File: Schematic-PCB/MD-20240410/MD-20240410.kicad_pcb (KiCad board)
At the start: 2 copper layers, 100.5 x 56.4 mm, 0 parts

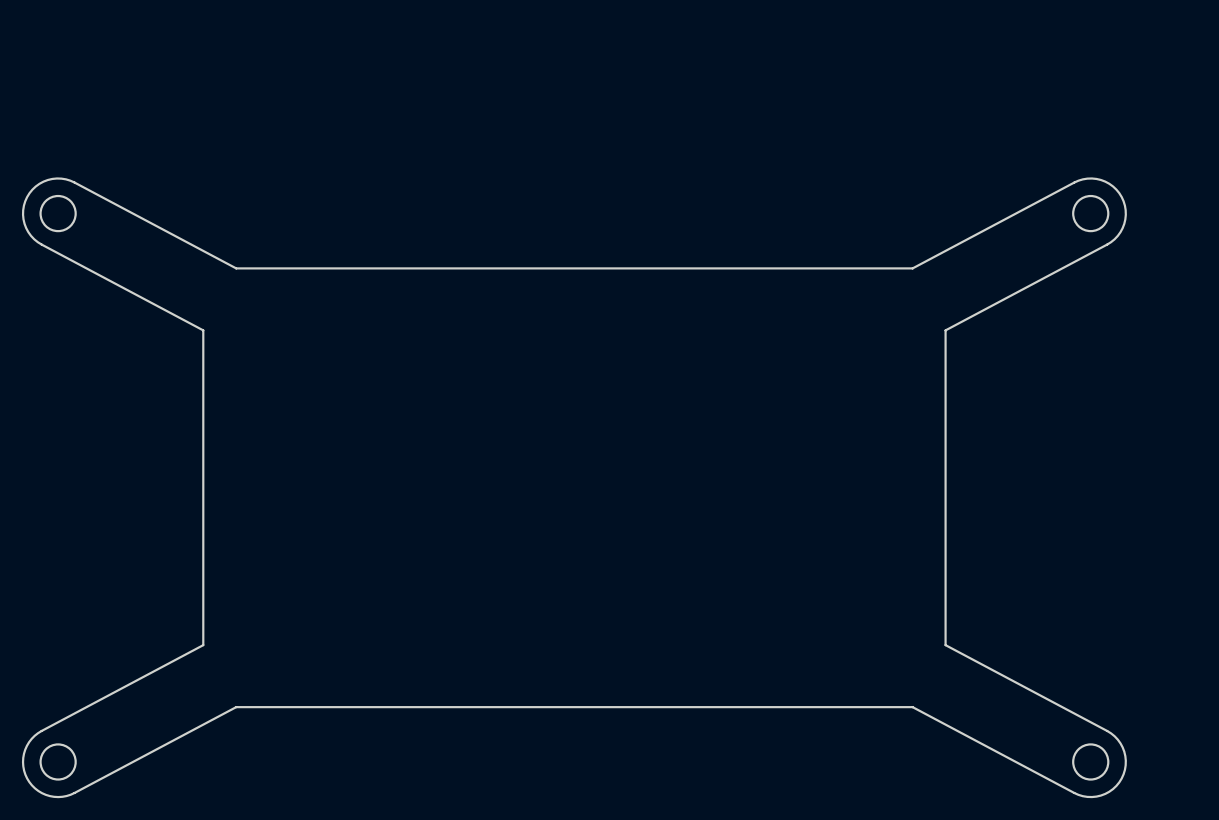
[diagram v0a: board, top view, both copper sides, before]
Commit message: MD基板へ部品を仮で配置
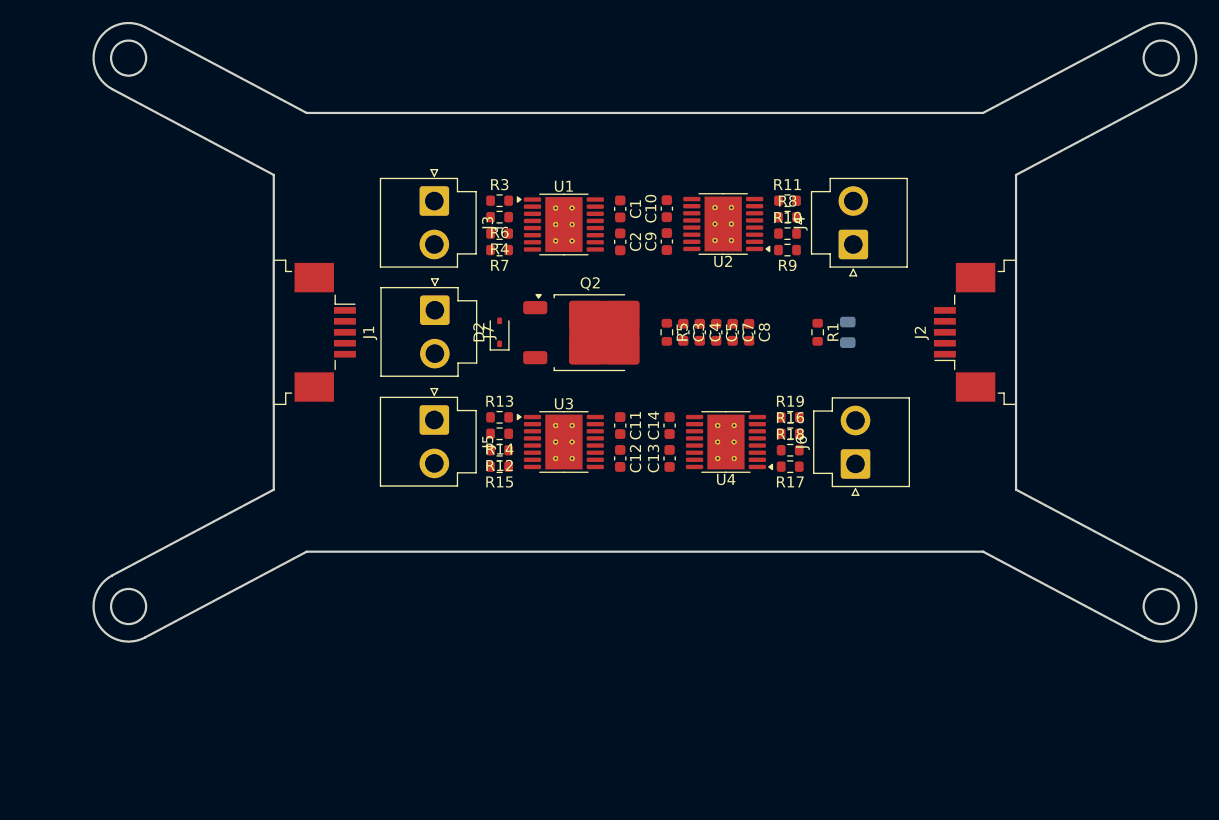
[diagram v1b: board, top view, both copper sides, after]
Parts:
- added C1: 22n, Capacitor_SMD:C_0603_1608Metric, F.Cu at (147.8, 76.2)
- added C10: 220n, Capacitor_SMD:C_0603_1608Metric, F.Cu at (152.0, 76.2)
- added C11: 22n, Capacitor_SMD:C_0603_1608Metric, F.Cu at (147.8, 96.0)
- added C12: 220n, Capacitor_SMD:C_0603_1608Metric, F.Cu at (147.8, 99.0)
- added C13: 22n, Capacitor_SMD:C_0603_1608Metric, F.Cu at (152.2, 99.0)
- added C14: 220n, Capacitor_SMD:C_0603_1608Metric, F.Cu at (152.2, 96.0)
- added C2: 220n, Capacitor_SMD:C_0603_1608Metric, F.Cu at (147.8, 79.2)
- added C3: 4.7u, Capacitor_SMD:C_0603_1608Metric, F.Cu at (153.5, 87.5)
- added C4: 4.7u, Capacitor_SMD:C_0603_1608Metric, F.Cu at (155.0, 87.5)
- added C5: 50u, Capacitor_SMD:C_0603_1608Metric, F.Cu at (156.5, 87.5)
- added C7: 0.1u, Capacitor_SMD:C_0603_1608Metric, F.Cu at (158.0, 87.5)
- added C8: 0.1u, Capacitor_SMD:C_0603_1608Metric, F.Cu at (159.5, 87.5)
- added C9: 22n, Capacitor_SMD:C_0603_1608Metric, F.Cu at (152.0, 79.2)
- added D1: LED, LED_SMD:LED_0805_2012Metric, B.Cu at (168.5, 87.5)
- added D2: 16.2V, Diode_SMD:D_SOD-323, F.Cu at (136.8, 87.5)
- added J1: Conn_01x05_Pin, Connector_FFC-FPC:TE_84953-5_1x05-1MP_P1.0mm_Horizontal, F.Cu at (120.8, 87.5)
- added J2: Conn_01x05_Pin, Connector_FFC-FPC:TE_84953-5_1x05-1MP_P1.0mm_Horizontal, F.Cu at (179.2, 87.5)
- added J3: Conn_01x02_Pin, Connector_JST:JST_VH_B2P-VH_1x02_P3.96mm_Vertical, F.Cu at (130.8, 75.5)
- added J4: Conn_01x02_Pin, Connector_JST:JST_VH_B2P-VH_1x02_P3.96mm_Vertical, F.Cu at (169.0, 79.5)
- added J5: Conn_01x02_Pin, Connector_JST:JST_VH_B2P-VH_1x02_P3.96mm_Vertical, F.Cu at (130.8, 95.5)
- added J6: Conn_01x02_Pin, Connector_JST:JST_VH_B2P-VH_1x02_P3.96mm_Vertical, F.Cu at (169.2, 99.5)
- added J7: Conn_01x02_Pin, Connector_JST:JST_VH_B2P-VH_1x02_P3.96mm_Vertical, F.Cu at (130.8, 85.5)
- added Q2: PMOS, Package_TO_SOT_SMD:TO-252-2, F.Cu at (145.0, 87.5)
- added R1: 330, Resistor_SMD:R_0603_1608Metric, F.Cu at (165.8, 87.5)
- added R10: NP, Resistor_SMD:R_0603_1608Metric, F.Cu at (163.0, 78.5)
- added R11: 20k, Resistor_SMD:R_0603_1608Metric, F.Cu at (163.0, 75.5)
- added R12: 2.49k, Resistor_SMD:R_0603_1608Metric, F.Cu at (136.8, 98.2)
- added R13: 10k, Resistor_SMD:R_0603_1608Metric, F.Cu at (136.8, 95.2)
- added R14: NP, Resistor_SMD:R_0603_1608Metric, F.Cu at (136.8, 96.8)
- added R15: 20k, Resistor_SMD:R_0603_1608Metric, F.Cu at (136.8, 99.8)
- added R16: 2.49k, Resistor_SMD:R_0603_1608Metric, F.Cu at (163.2, 96.8)
- added R17: 10k, Resistor_SMD:R_0603_1608Metric, F.Cu at (163.2, 99.8)
- added R18: NP, Resistor_SMD:R_0603_1608Metric, F.Cu at (163.2, 98.2)
- added R19: 20k, Resistor_SMD:R_0603_1608Metric, F.Cu at (163.2, 95.2)
- added R3: 10k, Resistor_SMD:R_0603_1608Metric, F.Cu at (136.8, 75.5)
- added R4: 2.49k, Resistor_SMD:R_0603_1608Metric, F.Cu at (136.8, 78.5)
- added R5: 100k, Resistor_SMD:R_0603_1608Metric, F.Cu at (152.0, 87.5)
- added R6: NP, Resistor_SMD:R_0603_1608Metric, F.Cu at (136.8, 77.0)
- added R7: 20k, Resistor_SMD:R_0603_1608Metric, F.Cu at (136.8, 80.0)
- added R8: 2.49k, Resistor_SMD:R_0603_1608Metric, F.Cu at (163.0, 77.0)
- added R9: 10k, Resistor_SMD:R_0603_1608Metric, F.Cu at (163.0, 80.0)
- added U1: ~, Package_SO:HTSSOP-16-1EP_4.4x5mm_P0.65mm_EP3.4x5mm_Mask2.46x2.31mm_ThermalVias, F.Cu at (142.6, 77.7)
- added U2: ~, Package_SO:HTSSOP-16-1EP_4.4x5mm_P0.65mm_EP3.4x5mm_Mask2.46x2.31mm_ThermalVias, F.Cu at (157.1, 77.6)
- added U3: ~, Package_SO:HTSSOP-16-1EP_4.4x5mm_P0.65mm_EP3.4x5mm_Mask2.46x2.31mm_ThermalVias, F.Cu at (142.6, 97.5)
- added U4: ~, Package_SO:HTSSOP-16-1EP_4.4x5mm_P0.65mm_EP3.4x5mm_Mask2.46x2.31mm_ThermalVias, F.Cu at (157.4, 97.5)
